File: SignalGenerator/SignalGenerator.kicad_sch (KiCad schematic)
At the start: 55 parts, among them J1 Buss PD, J2 AVR-ICSP, J3 I2C Display, J4 Conn_Coaxial, J5 Screw_Terminal_01x04, SW1 SW_Push_SPDT, T1 Transformer_1P_SS, U1 LM7805_TO220, U2 ATmega328P-AU, U3 LM7812_TO220, U4 LM7912_TO220, U5 AD8021, U6 AD9833BRMZ, X1 Oscillator, Y1 Crystal_cfpx-104

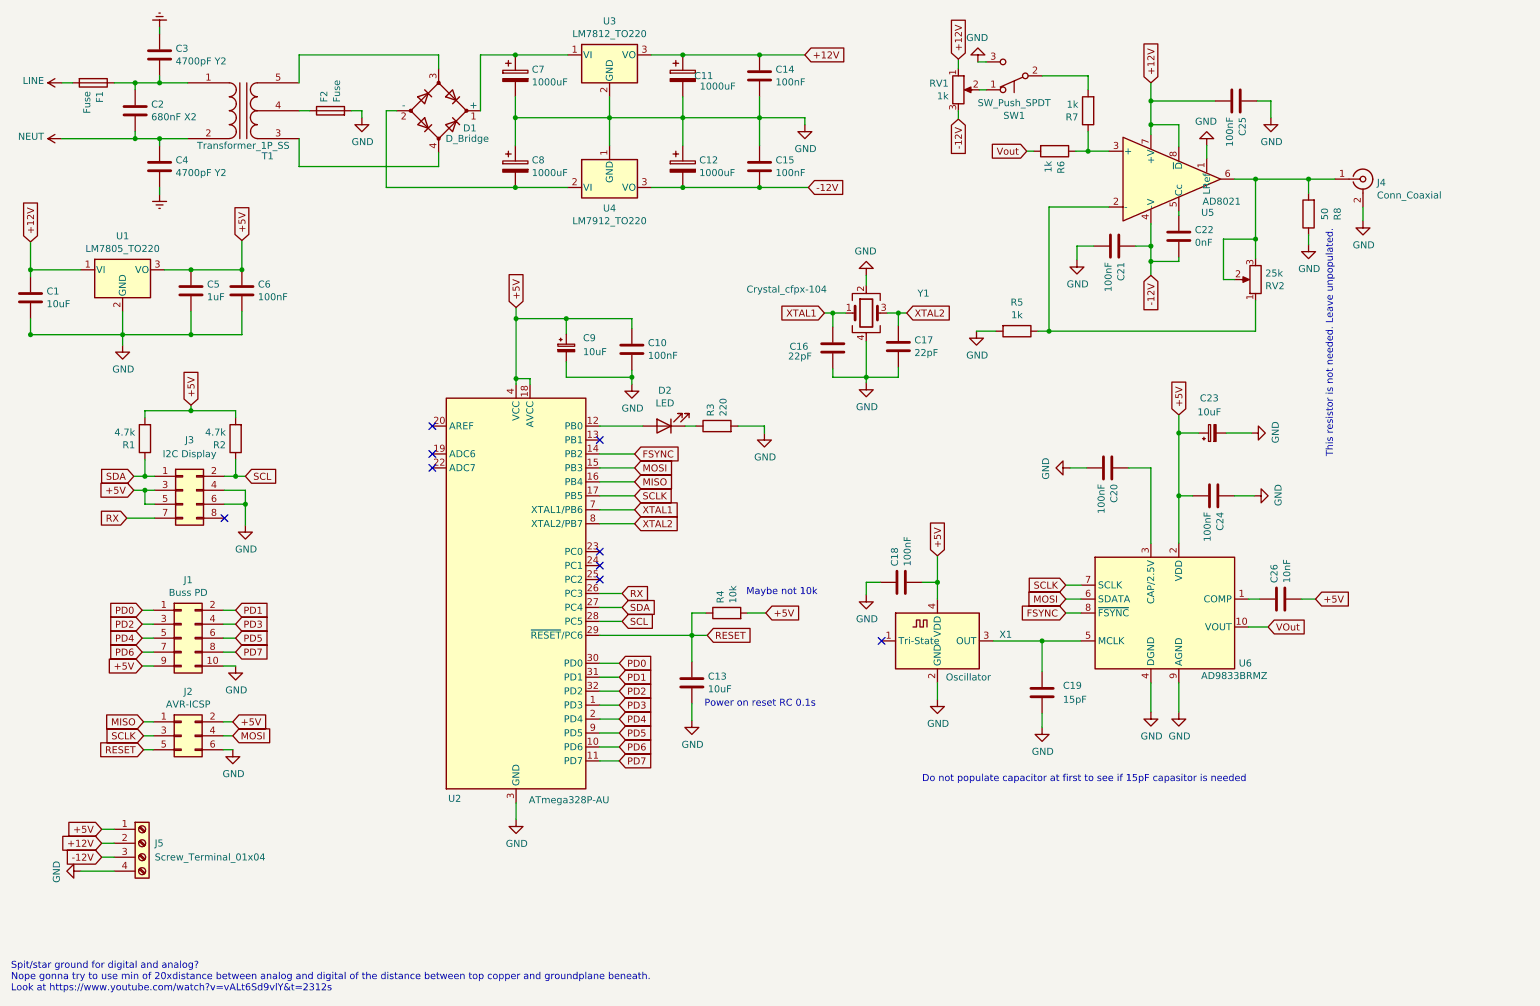
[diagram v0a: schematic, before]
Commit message: adf
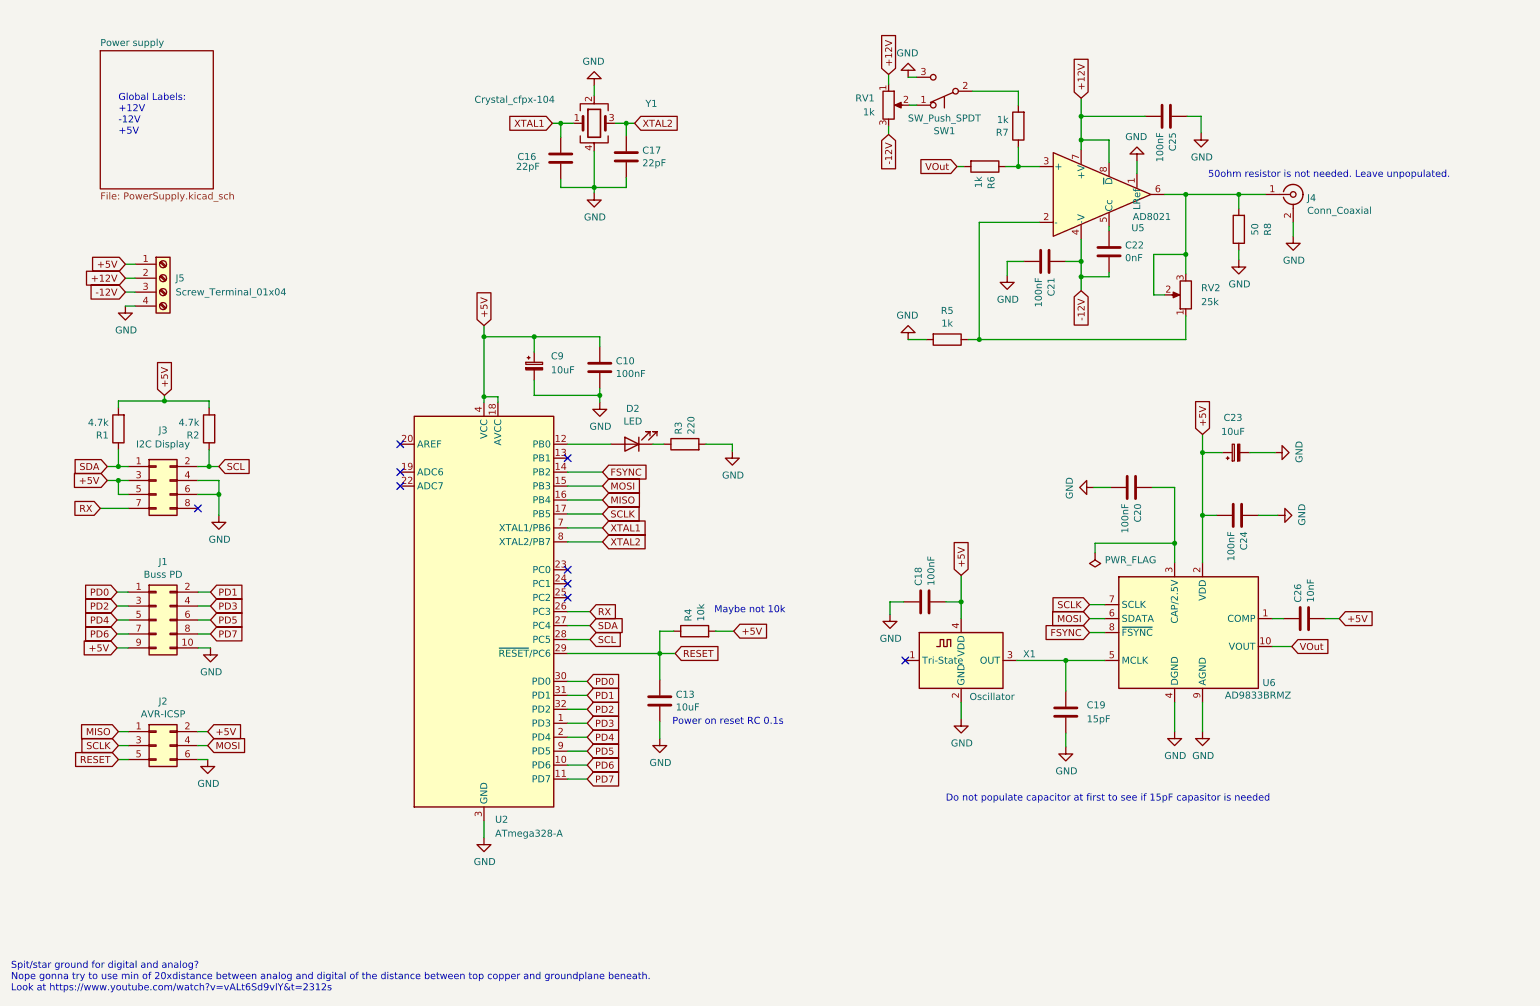
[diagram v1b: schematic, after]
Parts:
- removed C1: 10uF, Capacitor_SMD:C_1206_3216Metric_Pad1.33x1.80mm_HandSolder, symbol Device:C
- removed C11, C12, C7, C8: 1000uF, symbol Device:CP
- removed C14, C15: 100nF, symbol Device:C
- removed C2: 680nF X2, symbol Device:C
- removed C3, C4: 4700pF Y2, symbol Device:C
- removed C5: 1uF, Capacitor_SMD:C_0805_2012Metric_Pad1.18x1.45mm_HandSolder, symbol Device:C
- removed C6: 100nF, Capacitor_SMD:C_0805_2012Metric_Pad1.18x1.45mm_HandSolder, symbol Device:C
- removed D1: D_Bridge, symbol Device:D_Bridge_+-AA
- removed F1, F2: Fuse, symbol Device:Fuse
- removed RV1: 1k, Connector_PinHeader_2.54mm:PinHeader_1x03_P2.54mm_Vertical, symbol Device:R_POT
- removed RV2: 25k, Connector_PinHeader_2.54mm:PinHeader_1x03_P2.54mm_Vertical, symbol Device:R_POT
- removed T1: Transformer_1P_SS, symbol Device:Transformer_1P_SS
- removed U1: LM7805_TO220, Package_TO_SOT_THT:TO-220-3_Vertical, symbol Regulator_Linear:LM7805_TO220
- removed U2: ATmega328P-AU, Package_QFP:TQFP-32_7x7mm_P0.8mm, symbol MCU_Microchip_ATmega:ATmega328P-AU
- removed U3: LM7812_TO220, Package_TO_SOT_THT:TO-220-3_Vertical, symbol Regulator_Linear:LM7812_TO220
- removed U4: LM7912_TO220, Package_TO_SOT_THT:TO-220-3_Vertical, symbol Regulator_Linear:LM7912_TO220
- added RV1: 1k, symbol Device:R_Potentiometer
- added RV2: 25k, symbol Device:R_Potentiometer
- added U2: ATmega328-A, Package_QFP:TQFP-32_7x7mm_P0.8mm, symbol MCU_Microchip_ATmega:ATmega328-A
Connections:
- net Vout is gone; now on net VOut: R6.2
- net +12V: now also RV1.1
- net +5V: now also U2.18 (AVCC), U2.4 (VCC), U2.6 (VCC)
- net -12V: now also RV1.3
- net FSYNC: now also U2.14 (PB2)
- net GND: now also U2.21 (GND), U2.3 (GND), U2.5 (GND)
- net MISO: now also U2.16 (PB4)
- net MOSI: now also U2.15 (PB3)
- net PD0: now also U2.30 (PD0)
- net PD1: now also U2.31 (PD1)
- net PD2: now also U2.32 (PD2)
- net PD3: now also U2.1 (PD3)
- net PD4: now also U2.2 (PD4)
- net PD5: now also U2.9 (PD5)
- net PD6: now also U2.10 (PD6)
- net PD7: now also U2.11 (PD7)
- net RESET: now also U2.29 (~{RESET}/PC6)
- net RX: now also U2.26 (PC3)
- net SCL: now also U2.28 (PC5)
- net SCLK: now also U2.17 (PB5)
- net SDA: now also U2.27 (PC4)
- net XTAL1: now also U2.7 (XTAL1/PB6)
- net XTAL2: now also U2.8 (XTAL2/PB7)
- net at R5.1, U5.2 (-): now also RV2.1
- net at J4.1 (In), R8.2, U5.6: now also RV2.2, RV2.3
- net at SW1.1 (A): now also RV1.2
- net at D2.2 (A): now also U2.12 (PB0)
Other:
- added sheet Power supply (PowerSupply.kicad_sch)
- note added: "50ohm resistor is not needed. Leave unpopulated."
- note added: "Global Labels: +12V -12V +5V"
- note removed: "This resistor is not needed. Leave unpopulated."
- moved on the sheet: C10, C13, C16, C17, C18, C19, C20, C21, C22, C23, C24, C25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

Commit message: First real revision to the PCB done.
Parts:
- RV1, RV2: footprint (none) -> Connector_PinHeader_2.54mm:PinHeader_1x03_P2.54mm_Vertical
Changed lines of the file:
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@@
       (effects (font (size 1.27 1.27)) (justify right))
     )
-    (property "Footprint" "" (id 2) (at 229.362 66.548 0)
+    (property "Footprint" "Connector_PinHeader_2.54mm:PinHeader_1x03_P2.54mm_Vertical" (id 2) (at 229.362 66.548 0)
       (effects (font (size 1.27 1.27)) hide)
     )
@@
       (effects (font (size 1.27 1.27)) (justify right))
     )
-    (property "Footprint" "" (id 2) (at 175.26 32.004 0)
+    (property "Footprint" "Connector_PinHeader_2.54mm:PinHeader_1x03_P2.54mm_Vertical" (id 2) (at 175.26 32.004 0)
       (effects (font (size 1.27 1.27)) hide)
     )
@@
     )
     (path "/b56b0fa3-3e7f-4c85-bcf3-d61be9c95bdd"
-      (reference "RV1") (unit 1) (value "1k") (footprint "")
+      (reference "RV1") (unit 1) (value "1k") (footprint "Connector_PinHeader_2.54mm:PinHeader_1x03_P2.54mm_Vertical")
     )
     (path "/05ab5460-9dc3-448d-a9a8-4c16ae09a4eb"
-      (reference "RV2") (unit 1) (value "25k") (footprint "")
+      (reference "RV2") (unit 1) (value "25k") (footprint "Connector_PinHeader_2.54mm:PinHeader_1x03_P2.54mm_Vertical")
     )
     (path "/00000000-0000-0000-0000-0000618b491b"
